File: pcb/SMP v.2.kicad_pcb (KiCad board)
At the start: 2 copper layers, 114.7 x 58.7 mm, 23 parts, among them U1 Elite-C-keebio_without_bottom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

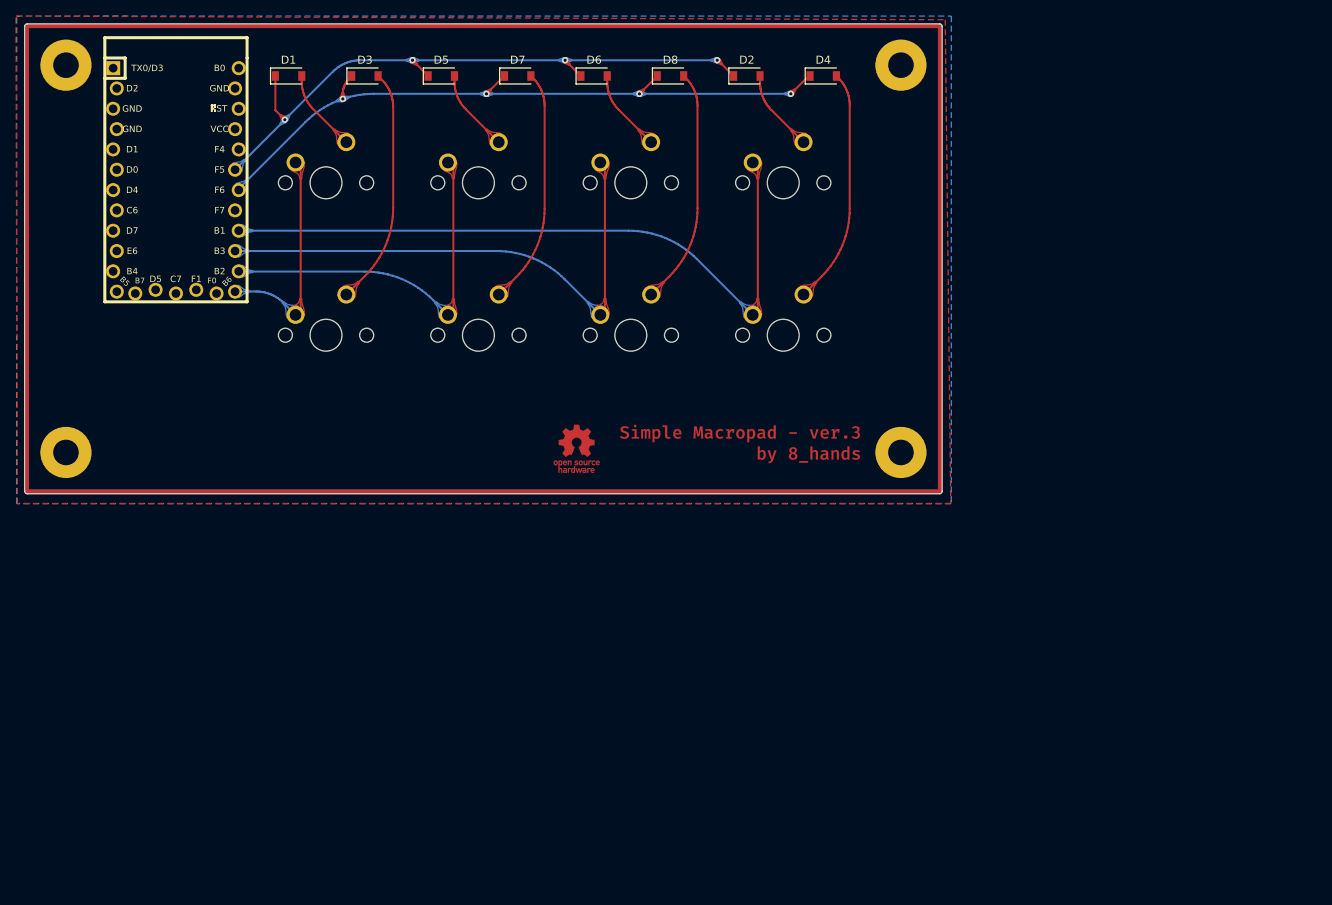
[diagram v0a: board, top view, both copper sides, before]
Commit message: pcb and plate finalize for v.4
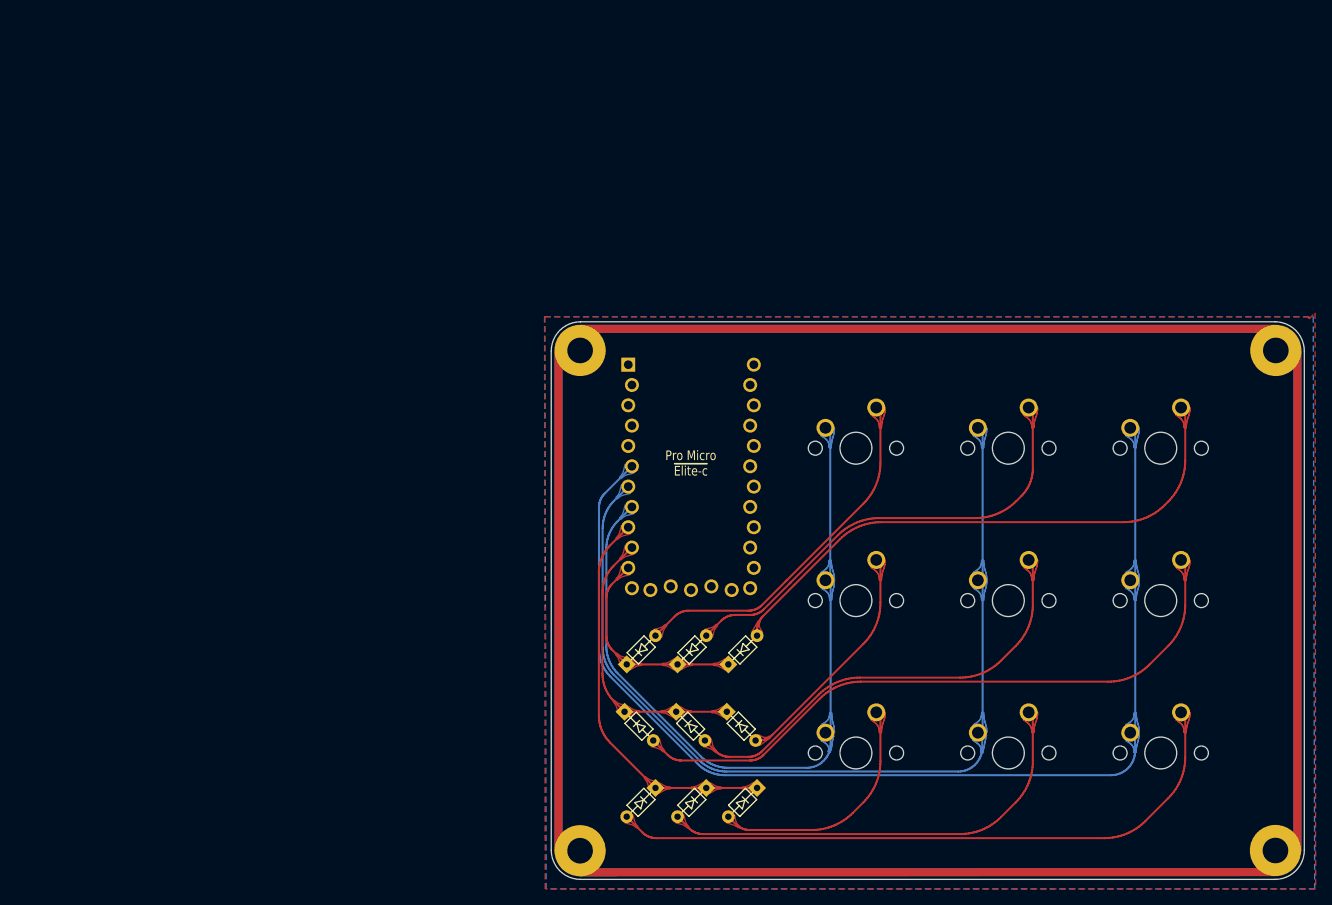
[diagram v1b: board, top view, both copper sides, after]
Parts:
- removed H1: MountingHole_Pad, MountingHole:MountingHole_3.2mm_M3_Pad
- removed REF**: OSHW-Logo_5.7x6mm_Copper, Symbol:OSHW-Logo_5.7x6mm_Copper
- removed Ref**: Val**, 8hands:smp_logo
- added D9: D_Small, 8hands:D_DO-35_SOD27_P5.08mm_Horizontal, F.Cu at (121.1, 119.8)
- added He: MountingHole_Pad, MountingHole:MountingHole_3.2mm_M3_Pad, F.Cu at (110.8, 66.0)
- added MX9: MX-NoLED, MX_Only:MXOnly-1U-NoLED, F.Cu at (183.4, 116.4)
- added kibuzzard-6147B285: G***, label, B.Cu at (183.9, 128.7)
- added kibuzzard-6147B2C4: G***, label, B.Cu at (186.7, 126.7)
- added kibuzzard-6147B3E3: G***, label, B.Cu at (178.7, 123.3)
- D1, D2, D3, D4, D5, D6, D7, D8: footprint Diode_SMD:D_SOD-123 -> 8hands:D_DO-35_SOD27_P5.08mm_Horizontal
- U1: footprint Keebio-Parts:Elite-C-ZigZag -> Keebio-Parts:Elite-C-ZigZag_no-fsilks
- moved H4 159.2 mm to (197.7, 128.5)
- moved H3 117.4 mm to (110.8, 128.6)
- moved D7 93.3 mm to (133.8, 119.8), turned to 225 degrees
- moved MX6 91.5 mm to (183.4, 97.3)
- moved MX5 91.5 mm to (164.3, 97.3)
- moved D8 88.3 mm to (127.5, 119.8), turned to 225 degrees
- moved D3 86.8 mm to (128.4, 106.2), turned to 45 degrees
- moved D1 85.2 mm to (115.7, 106.2), turned to 45 degrees
- moved D5 83.6 mm to (121.9, 110.3), turned to 315 degrees
- moved D4 79.6 mm to (128.2, 110.3), turned to 315 degrees
- moved D6 78.6 mm to (115.5, 110.3), turned to 315 degrees
- moved D2 75.1 mm to (122.1, 106.2), turned to 45 degrees
- moved U1 74.3 mm to (124.7, 81.8)
- moved MX1 74.1 mm to (145.3, 78.3)
- moved MX2 74.1 mm to (164.3, 78.3)
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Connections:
- D1 pad 1: ROW1 -> ROW2
- D2 pad 1: ROW1 -> ROW2
- D3 pad 1: ROW0 -> ROW2
- D4 pad 1: ROW0 -> ROW1
- MX2 pad 2: Net-(D5-Pad2) -> Net-(D2-Pad2)
- MX3 pad 2: Net-(D6-Pad2) -> Net-(D3-Pad2)
- MX4 pad 1: COL3 -> COL0
- MX4 pad 2: Net-(D2-Pad2) -> Net-(D4-Pad2)
- MX5 pad 1: COL0 -> COL1
- MX5 pad 2: Net-(D3-Pad2) -> Net-(D5-Pad2)
- MX6 pad 1: COL1 -> COL2
- MX6 pad 2: Net-(D7-Pad2) -> Net-(D6-Pad2)
- MX7 pad 1: COL2 -> COL0
- MX7 pad 2: Net-(D8-Pad2) -> Net-(D7-Pad2)
- MX8 pad 1: COL3 -> COL1
- MX8 pad 2: Net-(D4-Pad2) -> Net-(D8-Pad2)
- U1 pad 10: Net-(U1-Pad10) -> ROW1
- U1 pad 11: Net-(U1-Pad11) -> ROW2
- U1 pad 13: COL0 -> Net-(U1-Pad13)
- U1 pad 14: COL1 -> Net-(U1-Pad14)
- U1 pad 15: COL2 -> Net-(U1-Pad15)
- U1 pad 16: COL3 -> Net-(U1-Pad16)
- U1 pad 18: ROW0 -> Net-(U1-Pad18)
- U1 pad 19: ROW1 -> Net-(U1-Pad19)
- U1 pad 6: Net-(U1-Pad6) -> COL2
- U1 pad 7: Net-(U1-Pad7) -> COL1
- U1 pad 8: Net-(U1-Pad8) -> COL0
- U1 pad 9: Net-(U1-Pad9) -> ROW0
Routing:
- net COL3: track 87.7 -> 0.00 mm
- net Net-(D9-Pad2): track 0.00 -> 82.0 mm
- net COL2: track 68.6 -> 142.2 mm
- net Net-(D6-Pad2): track 10.3 -> 82.0 mm
- net COL1: track 47.5 -> 118.7 mm
- net COL0: track 28.2 -> 97.5 mm
- net Net-(D2-Pad2): track 10.3 -> 57.6 mm
- net Net-(D5-Pad2): track 10.4 -> 56.1 mm
- net ROW1: track 80.1 -> 35.6 mm, vias 4 -> 0
- net Net-(D3-Pad2): track 29.8 -> 71.1 mm
- net ROW0: track 86.5 -> 49.3 mm, vias 4 -> 0
- net Net-(D1-Pad2): track 10.4 -> 45.6 mm
- net ROW2: track 0.00 -> 26.7 mm
- net Net-(D8-Pad2): track 29.7 -> 56.4 mm
- net Net-(D7-Pad2): track 29.7 -> 30.6 mm
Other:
- board size 114.7 x 58.7 mm -> 94.1 x 69.7 mm
- board text added: "Pro Micro ~Elite-c~"
- board text added: "rev.4"

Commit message: last commit
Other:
- net class Default removed
- net class Power removed
- board text added: "Pro Micro ~{Elite-c}"
- board text removed: "Pro Micro ~Elite-c~"
